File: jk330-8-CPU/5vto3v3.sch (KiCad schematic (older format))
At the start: 12 parts, among them U2 74LVCC3245, U3 74LVCC3245, U4 PCA9306, U6 74LVCC3245

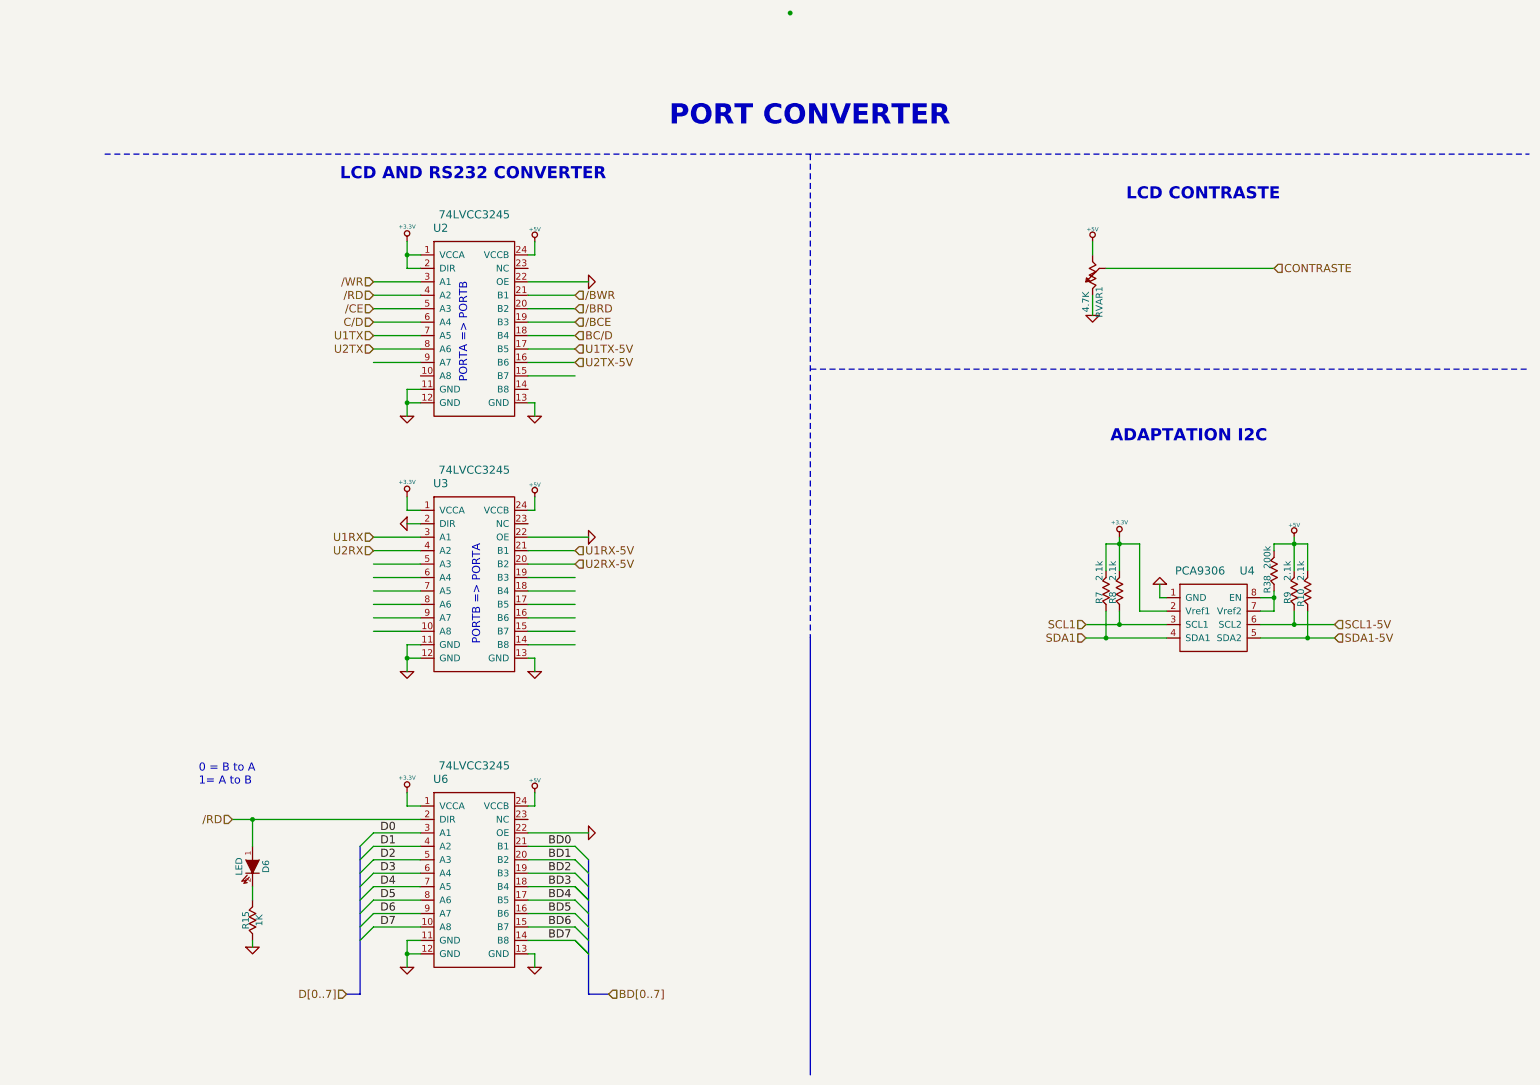
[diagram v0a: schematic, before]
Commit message: MAJ CPU
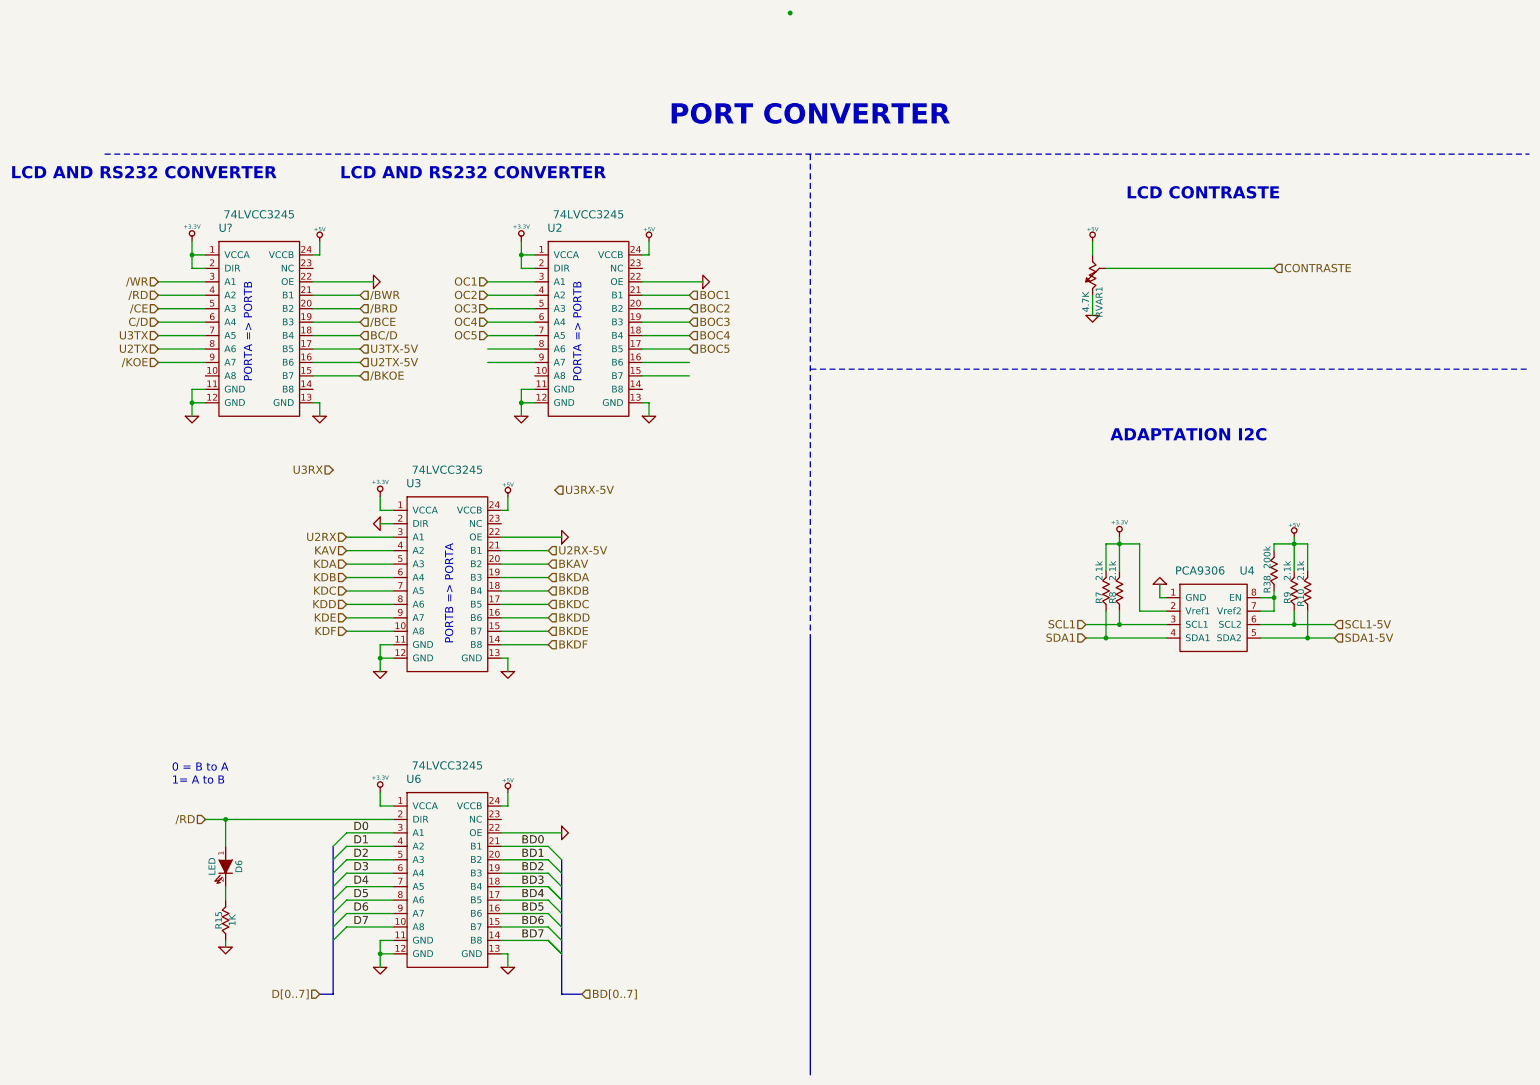
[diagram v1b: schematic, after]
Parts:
- added U?: 74LVCC3245, symbol 74LVCC3245
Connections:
- net labels added: /BKOE, /KOE, BKAV, BKDA, BKDB, BKDC, BKDD, BKDE, BKDF, BOC1, BOC2, BOC3, BOC4, BOC5, KAV, KDA, KDB, KDC, KDD, KDE, KDF, OC1, OC2, OC3, OC4, OC5, U3RX, U3RX-5V, U3TX, U3TX-5V
- net labels removed: U1RX, U1RX-5V, U1TX, U1TX-5V
- wire segments 107 -> 132
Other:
- moved on the sheet: D6, R15, U2, U3, U6
